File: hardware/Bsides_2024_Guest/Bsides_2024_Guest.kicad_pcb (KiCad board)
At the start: 2 copper layers, 134.5 x 127.4 mm, 40 parts, among them J1 Conn_02x03_Odd_Even, J2 Battery, J3 Battery, J4 OLED, P1 USB_C_Plug_USB2.0, Q1 DMG3415U-7, SW1 ON, SW2 RESET, SW3 BOOT, SW4 RESET, SW6 RESET, U1 ESP32-C6-WROOM-1U-N4, U2 AP2112K-3.3

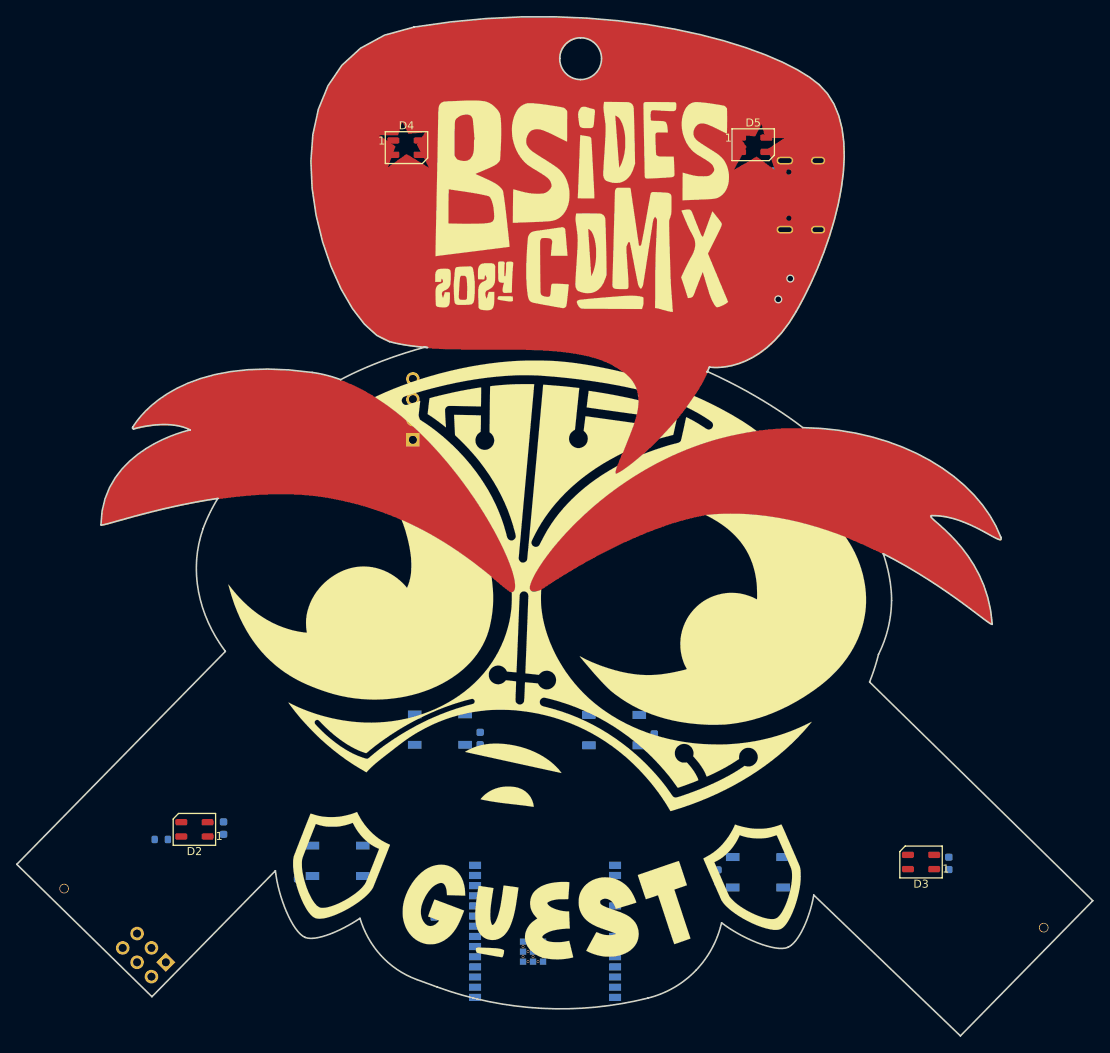
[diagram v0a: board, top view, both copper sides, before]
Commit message: feat(Hw): Shitty Addon PCB added
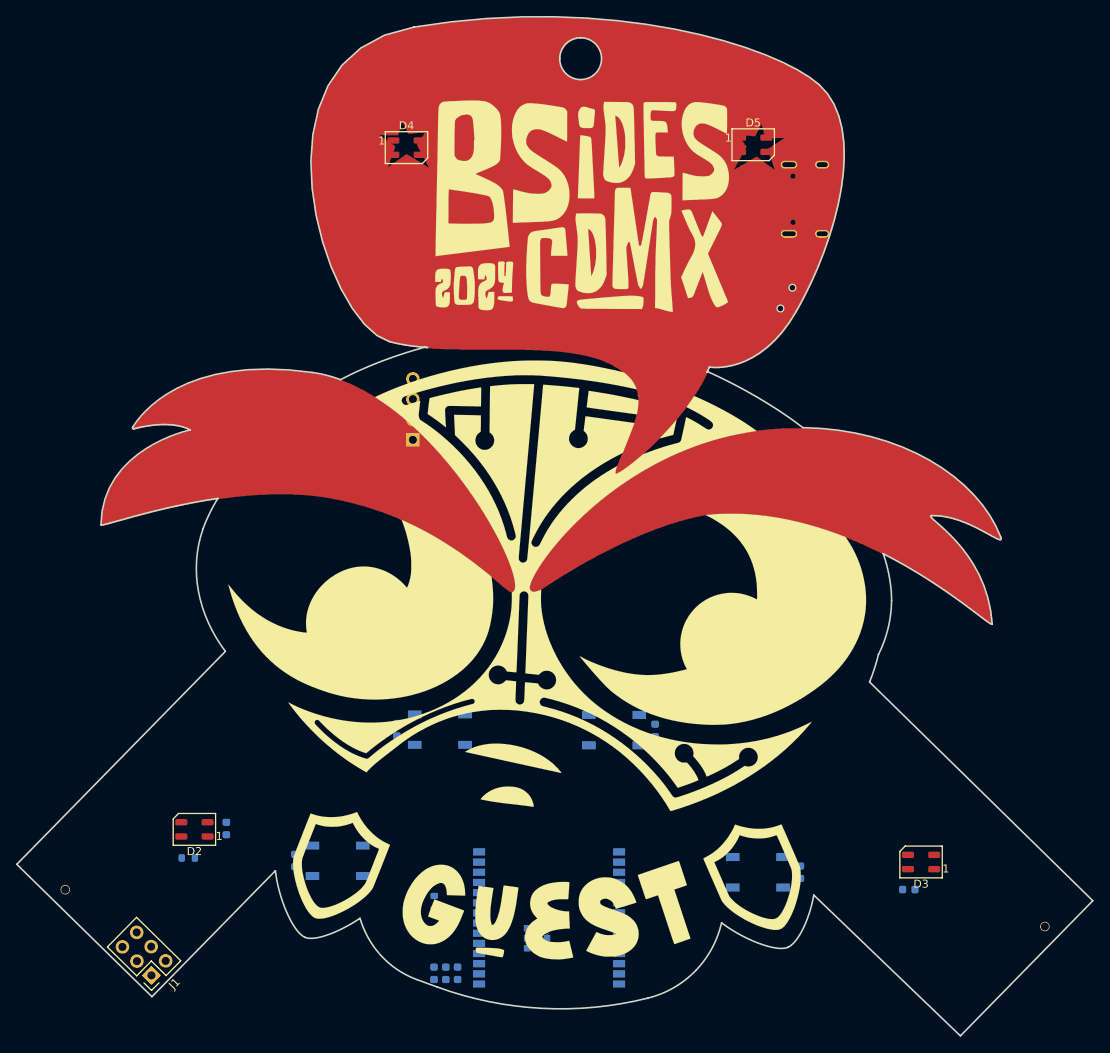
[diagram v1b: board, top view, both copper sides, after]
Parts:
- added C13: 1uF, Capacitor_SMD:C_0603_1608Metric, B.Cu at (113.3, 145.6)
- added C14: 10uF, Capacitor_SMD:C_0603_1608Metric, B.Cu at (111.9, 145.6)
- added C15: 10uF, Capacitor_SMD:C_0603_1608Metric, B.Cu at (110.4, 145.6)
- J1: moved to F.Cu
- moved C10 10.5 mm to (105.8, 115.1)
- moved C11 10.3 mm to (156.2, 133.0)
- moved C3 8.02 mm to (162.2, 85.6), turned to -90 degrees
- moved C6 5.97 mm to (169.8, 135.1), turned to 0 degrees
- moved R2 4.79 mm to (145.2, 56.2), turned to 0 degrees
- moved R6 4.09 mm to (79.7, 131.2), turned to 180 degrees
- moved R4 3.91 mm to (149.0, 50.6)
- moved Q1 3.50 mm to (143.5, 59.2), turned to 180 degrees
- moved D1 2.83 mm to (146.6, 59.2)
- moved R1 2.71 mm to (110.4, 136.8)
- moved C2 2.64 mm to (140.9, 65.2)
- moved U2 2.55 mm to (143.9, 65.4)
- moved J1 2.43 mm to (75.1, 145.8), turned to -134.5 degrees
- moved C1 2.42 mm to (146.8, 65.2)
- moved U1 1.74 mm to (124.8, 141.7)
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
